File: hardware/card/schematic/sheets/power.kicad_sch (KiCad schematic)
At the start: 9 parts, among them J1 USB-C-mid, J2 1S-Pouch-503048/603048, U2 BQ24075RGTR, U3 MAX17048G+T10, U4 TPS63070

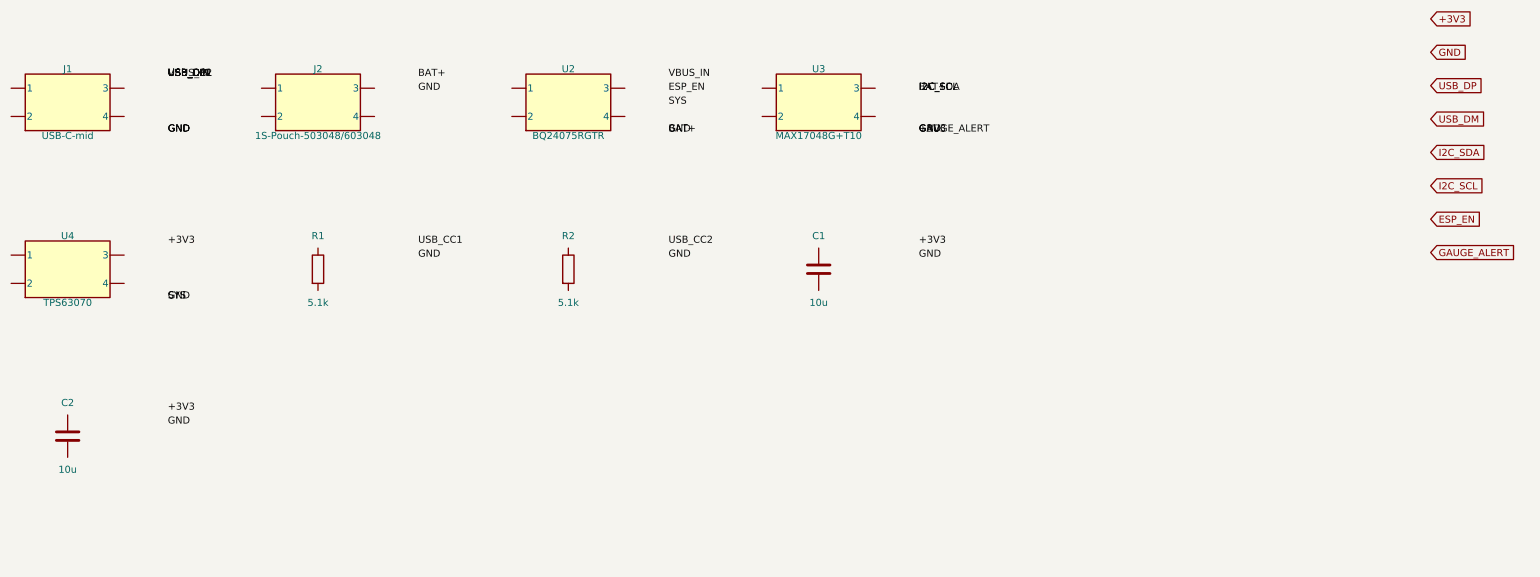
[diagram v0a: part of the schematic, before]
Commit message: pcb stuff
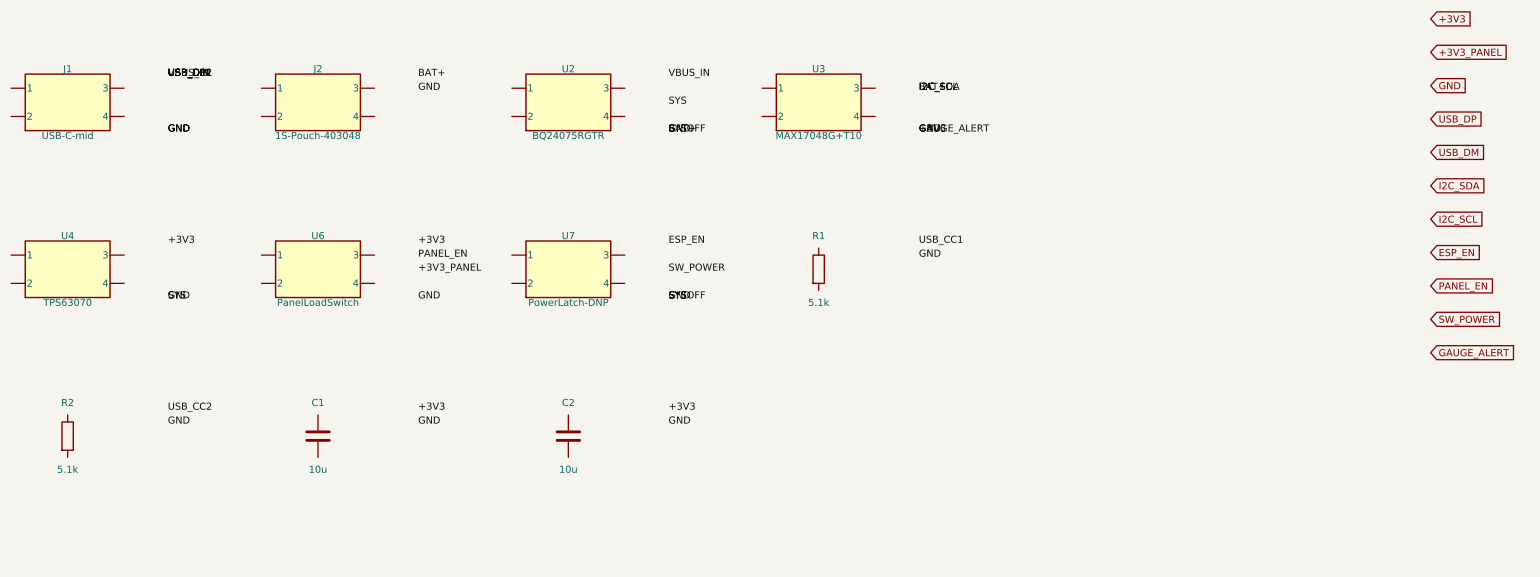
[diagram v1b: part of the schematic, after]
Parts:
- added R1: 5.1k, 0402, symbol Device:R
- added U7: PowerLatch-DNP, TBD, symbol PSCard:Block2
- J2: value 1S-Pouch-503048/603048 -> 1S-Pouch-403048
- U6: renamed from R1; value 5.1k -> PanelLoadSwitch; footprint 0402 -> TBD; symbol Device:R -> PSCard:Block2
